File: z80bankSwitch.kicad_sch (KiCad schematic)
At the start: 27 parts, among them J1 Conn_02x05_Odd_Even, P101 Conn_01x06_Pin, P102 Conn_02x20_Odd_Even, U1 SST39SF040, U101 7400, U102 Z8400, U105 74LS138, U3 EPM3032A, U4 AS6C8008-55ZIN, Y101 Crystal

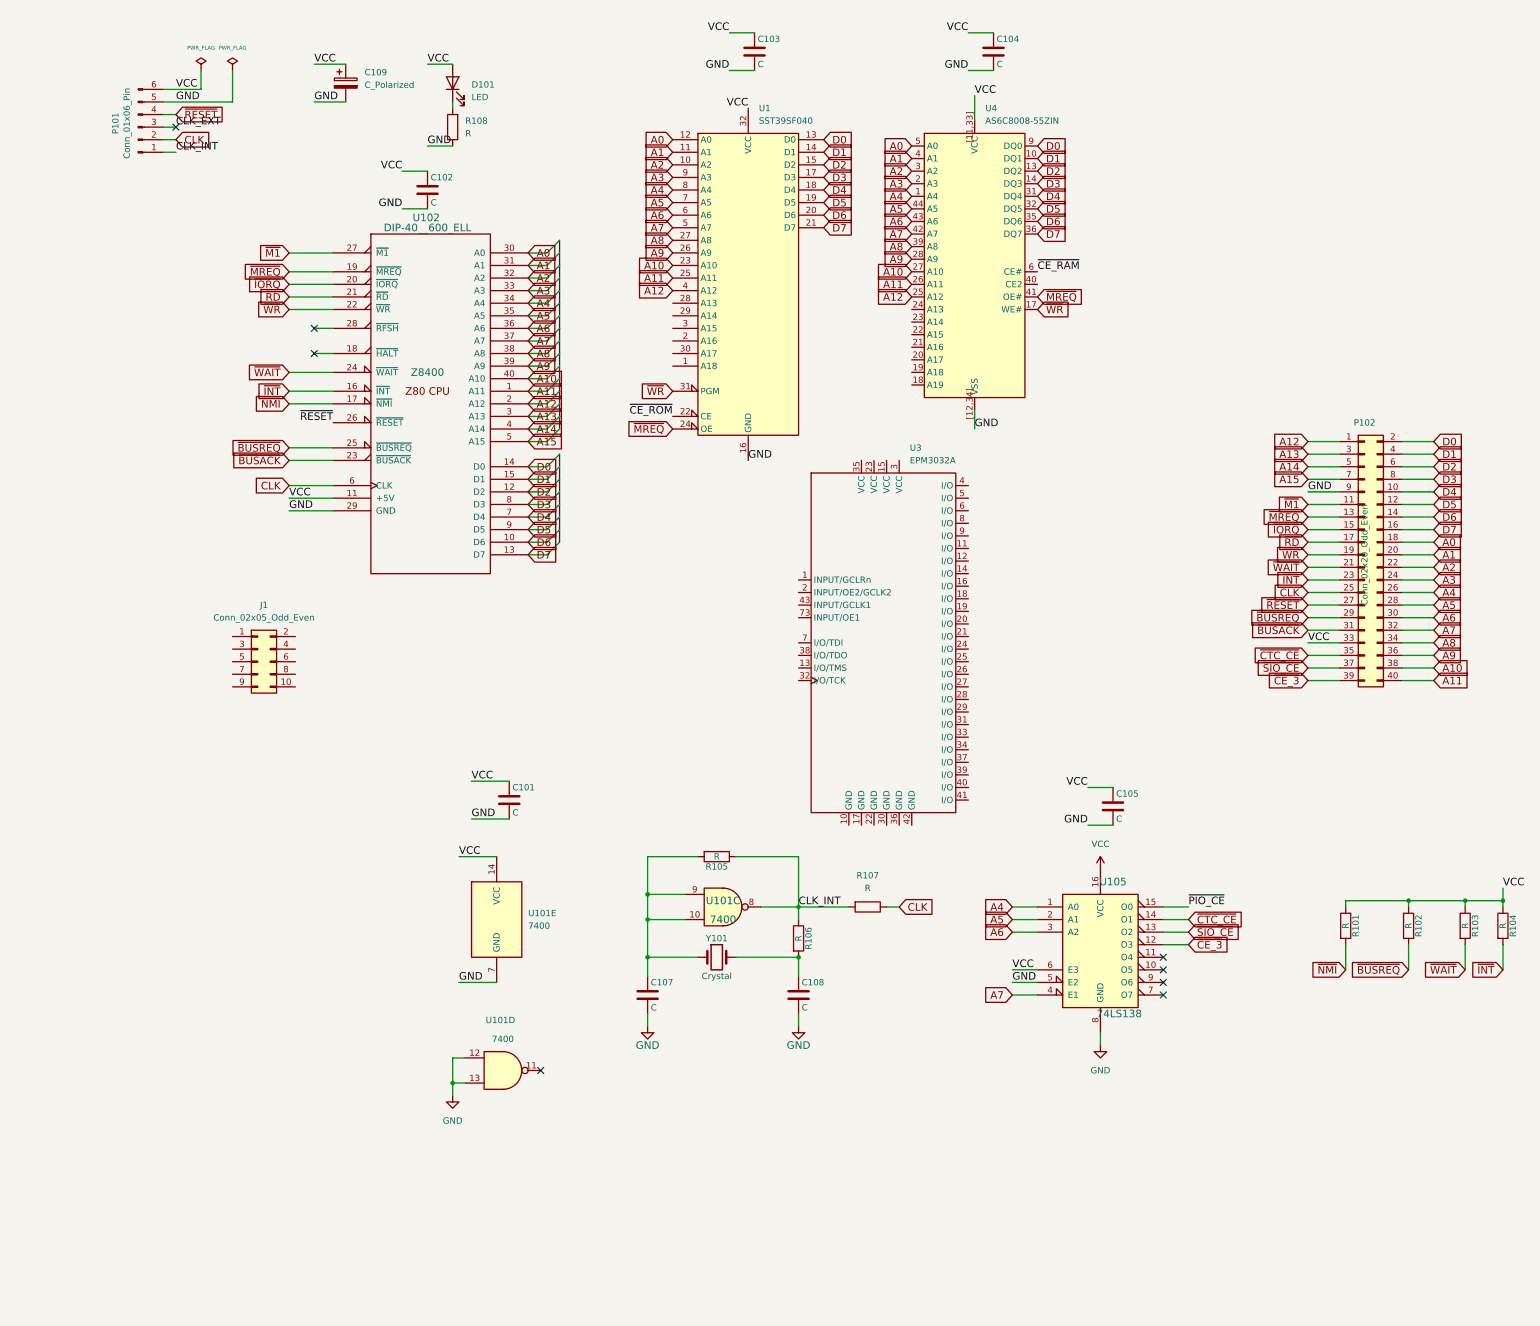
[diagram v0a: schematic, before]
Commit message: Schematics mostly wired
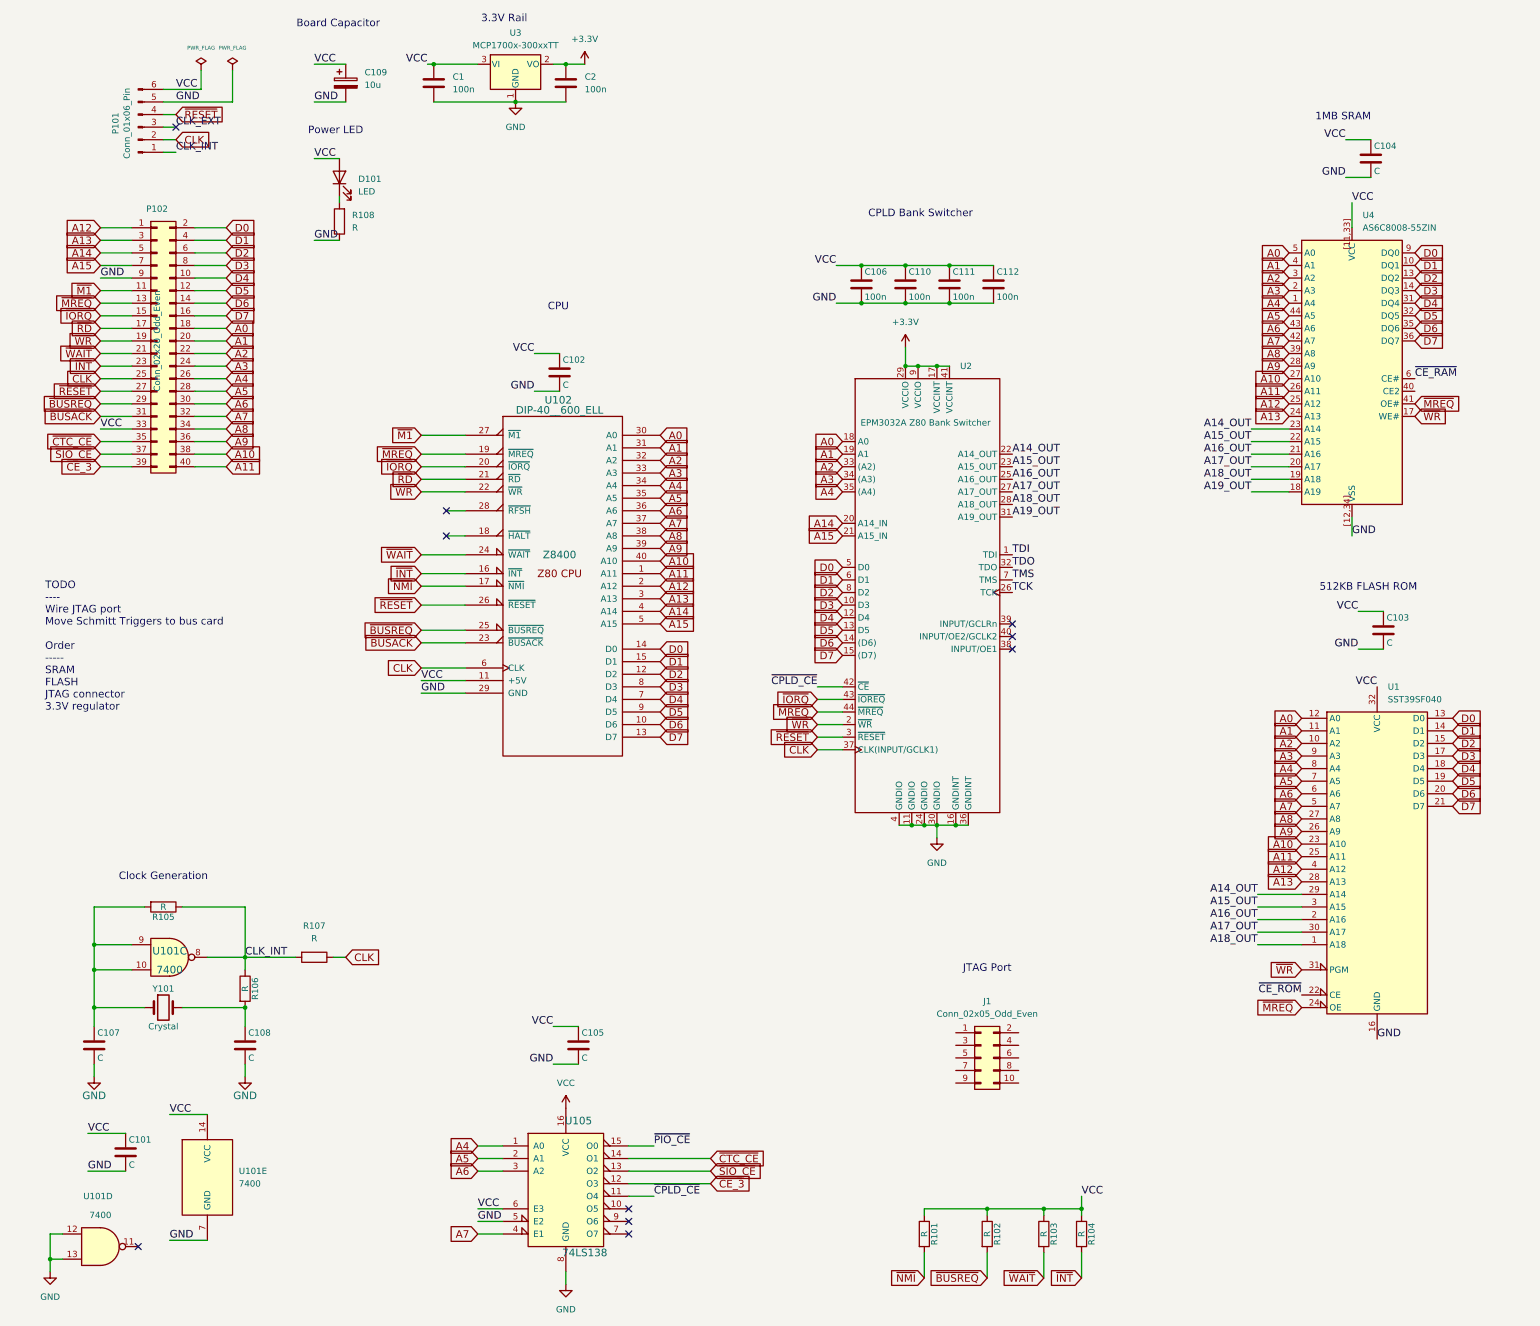
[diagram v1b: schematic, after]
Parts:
- removed U3: EPM3032A, Package_QFP:TQFP-44_10x10mm_P0.8mm, symbol Own Symbol Library:EPM3032A
- added C1, C106, C110, C111, C112, C2: 100n, Capacitor_SMD:C_0805_2012Metric_Pad1.18x1.45mm_HandSolder, symbol Device:C
- added U2: EPM3032A Z80 Bank Switcher, Package_QFP:TQFP-44_10x10mm_P0.8mm, symbol Own Symbol Library:EPM3032A_Z80_Bank_Switcher
- added U3: MCP1700x-300xxTT, Package_TO_SOT_SMD:SOT-23, symbol Regulator_Linear:MCP1700x-300xxTT
- C109: value C_Polarized -> 10u
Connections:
- net A0: now also U2.18 (A0)
- net A1: now also U2.19 (A1)
- net A13: now also U1.28 (A13), U4.24 (A13)
- net A14: now also U2.20 (A14_IN)
- net A15: now also U2.21 (A15_IN)
- net A2: now also U2.33 ((A2))
- net A3: now also U2.34 ((A3))
- net A4: now also U2.35 ((A4))
- net CLK: now also U2.37 (CLK(INPUT/GCLK1))
- net D0: now also U2.5 (D0)
- net D1: now also U2.6 (D1)
- net D2: now also U2.8 (D2)
- net D3: now also U2.10 (D3)
- net D4: now also U2.12 (D4)
- net D5: now also U2.13 (D5)
- net D6: now also U2.14 ((D6))
- net D7: now also U2.15 ((D7))
- net GND: now also C1.2, C106.2, C110.2, C111.2, C112.2, C2.2, U2.11 (GNDIO), U2.16 (GNDINT), U2.24 (GNDIO), U2.30 (GNDIO), U2.36 (GNDINT), U2.4 (GNDIO), U3.1 (GND)
- net VCC: now also C1.1, C106.1, C110.1, C111.1, C112.1, U3.3 (VI)
- net ~{IORQ}: now also U2.43 (~{IOREQ})
- net ~{MREQ}: now also U2.44 (~{MREQ})
- net ~{RESET}: now also U2.3 (~{RESET})
- net ~{WR}: now also U2.2 (~{WR})
- net ~{CPLD_CE}: now reaches U105.11 (O4)
- net ~{CPLD_CE}: now also U2.42 (~{CE})
- net A19_OUT: now reaches U4.18 (A19)
- net A19_OUT: now also U2.31 (A19_OUT)
- net A18_OUT: now reaches U4.19 (A18)
- net A18_OUT: now also U1.1 (A18), U2.28 (A18_OUT)
- net A17_OUT: now reaches U4.20 (A17)
- net A17_OUT: now also U1.30 (A17), U2.27 (A17_OUT)
- net A16_OUT: now reaches U4.21 (A16)
- net A16_OUT: now also U1.2 (A16), U2.25 (A16_OUT)
- net A15_OUT: now reaches U4.22 (A15)
- net A15_OUT: now also U1.3 (A15), U2.23 (A15_OUT)
- net A14_OUT: now reaches U4.23 (A14)
- net A14_OUT: now also U1.29 (A14), U2.22 (A14_OUT)
- new net +3.3V: C2.1, U2.17 (VCCINT), U2.29 (VCCIO), U2.41 (VCCINT), U2.9 (VCCIO), U3.2 (VO)
- new net TCK: U2.26 (TCK)
- new net TDI: U2.1 (TDI)
- new net TDO: U2.32 (TDO)
- new net TMS: U2.7 (TMS)
- no-connect marks 8 -> 10
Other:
- note added: "1MB SRAM"
- note added: "3.3V Rail"
- note added: "512KB FLASH ROM"
- note added: "Board Capacitor"
- note added: "CPLD Bank Switcher"
- note added: "CPU"
- note added: "Clock Generation"
- note added: "JTAG Port"
- note added: "Power LED"
- note added: "TODO ---- Wire JTAG port Move Schmitt Triggers to bus card Order ----- SRAM FLASH JTAG connector 3.3V regulator"
- moved on the sheet: C101, C102, C103, C104, C105, C107, C108, D101, J1, P102, R101, R102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
